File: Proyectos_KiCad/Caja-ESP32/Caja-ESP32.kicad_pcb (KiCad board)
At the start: 2 copper layers, 198 x 83 mm, 87 parts, among them J1 JACK_DC, J10 LOAD, J12 LOAD, J14 LOAD, J2 Fichero, J3 LOAD, J7 LOAD, J8 LOAD, Q1 TIP122, Q2 BT136-800, Q3 BT136-800, Q4 BT136-800, Q5 BT136-800, SW1 DIP_X06, U1 MP1584, U10 ESP32_DevKit_V1_DOIT, U2 AMS1117-3.3, U4 PC817, U5 PC817, U6 MOC3021M, U7 MOC3021M, U8 MOC3021M, U9 MOC3021M

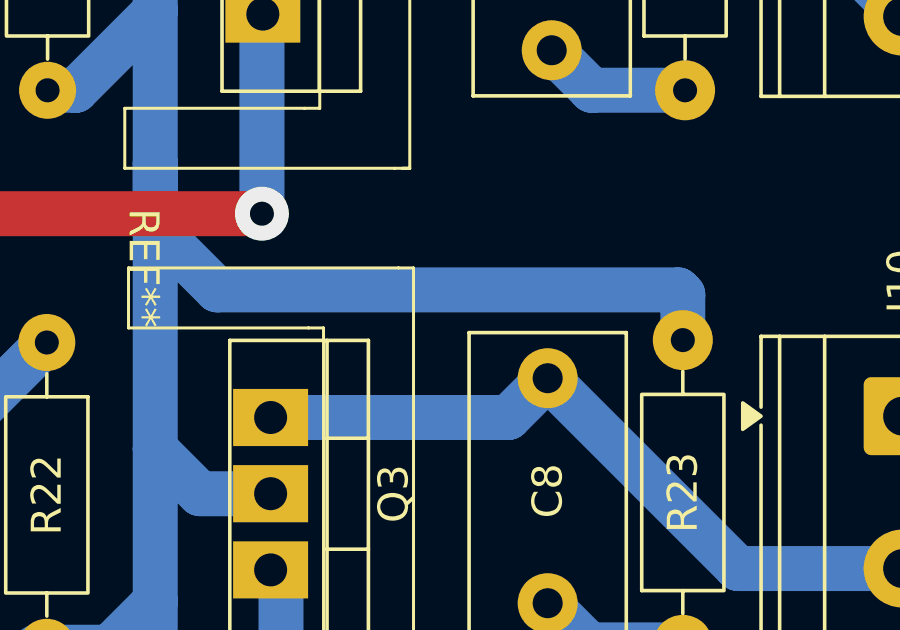
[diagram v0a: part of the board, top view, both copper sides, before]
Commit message: Hola
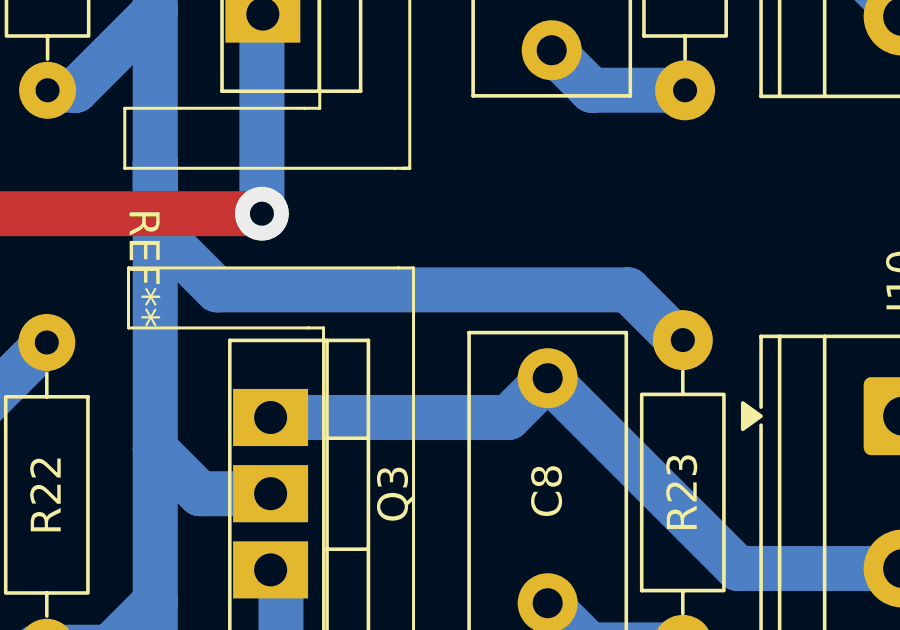
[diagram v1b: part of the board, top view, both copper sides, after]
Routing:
- net AC_1: track 195.8 -> 194.9 mm
